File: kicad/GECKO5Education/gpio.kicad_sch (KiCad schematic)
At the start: 3 parts, among them J6 M20-7920642R, J8 M20-7920642R, U6 LFE5U-85F-6BG381x

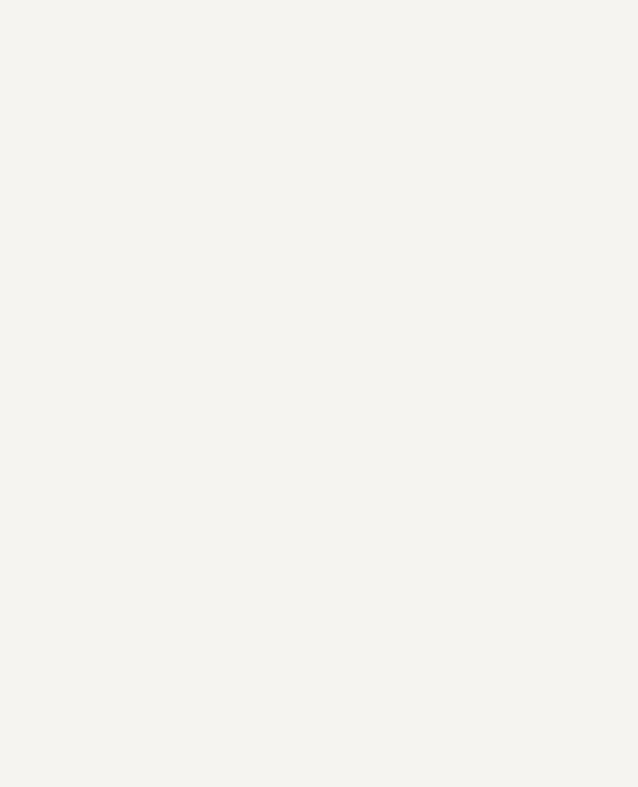
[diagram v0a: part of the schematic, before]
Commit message: Prototype Version V3.0
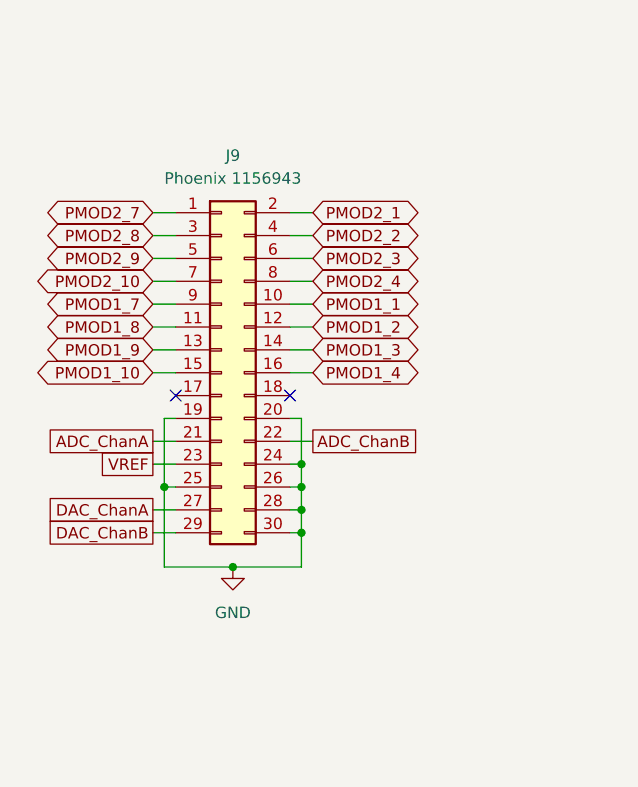
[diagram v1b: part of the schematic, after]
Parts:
- added J9: Phoenix 1156943, gecko4education:PHOENIX_1156943, symbol Connector_Generic:Conn_02x15_Odd_Even
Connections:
- net GND: now also J9.19 (Pin_19), J9.20 (Pin_20), J9.24 (Pin_24), J9.25 (Pin_25), J9.26 (Pin_26), J9.28 (Pin_28), J9.30 (Pin_30)
- net PMOD1_1: now also J9.10 (Pin_10)
- net PMOD1_10: now also J9.15 (Pin_15)
- net PMOD1_2: now also J9.12 (Pin_12)
- net PMOD1_3: now also J9.14 (Pin_14)
- net PMOD1_4: now also J9.16 (Pin_16)
- net PMOD1_7: now also J9.9 (Pin_9)
- net PMOD1_8: now also J9.11 (Pin_11)
- net PMOD1_9: now also J9.13 (Pin_13)
- net PMOD2_1: now also J9.2 (Pin_2)
- net PMOD2_10: now also J9.7 (Pin_7)
- net PMOD2_2: now also J9.4 (Pin_4)
- net PMOD2_3: now also J9.6 (Pin_6)
- net PMOD2_4: now also J9.8 (Pin_8)
- net PMOD2_7: now also J9.1 (Pin_1)
- net PMOD2_8: now also J9.3 (Pin_3)
- net PMOD2_9: now also J9.5 (Pin_5)
- new net ADC_ChanA: J9.21 (Pin_21)
- new net ADC_ChanB: J9.22 (Pin_22)
- new net DAC_ChanA: J9.27 (Pin_27)
- new net DAC_ChanB: J9.29 (Pin_29)
- new net VREF: J9.23 (Pin_23)
- no-connect marks 0 -> 2
